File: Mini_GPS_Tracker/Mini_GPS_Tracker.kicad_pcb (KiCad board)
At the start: 2 copper layers, 34 parts, among them J1 USB_C_Receptacle, J2 5-1814400-1, J3 XT60-M, SW1 SW_Push, U1 CH340E, U2 XBee_SMT, U3 MAX-8Q, U4 LD1117S33TR_SOT223, U5 MS5611-01BA, Y1 Crystal

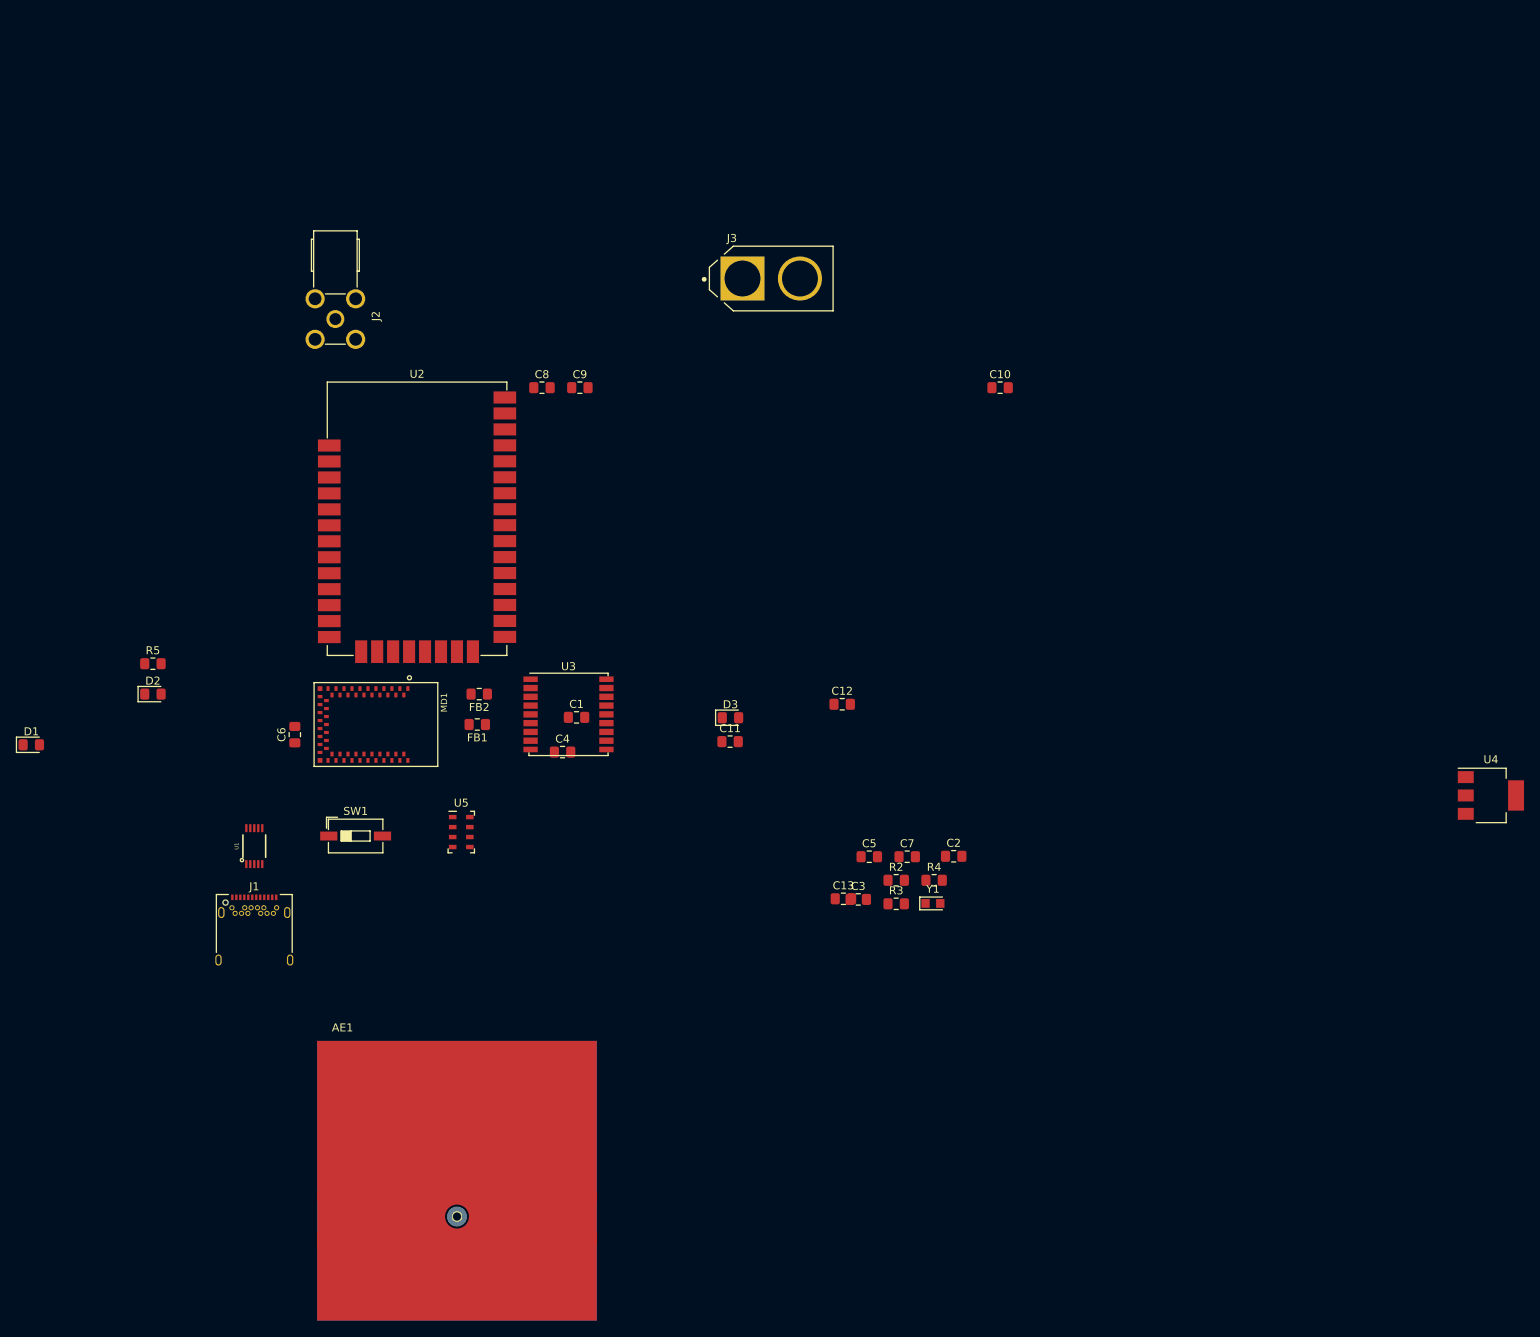
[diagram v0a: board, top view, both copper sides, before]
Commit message: worked on routing
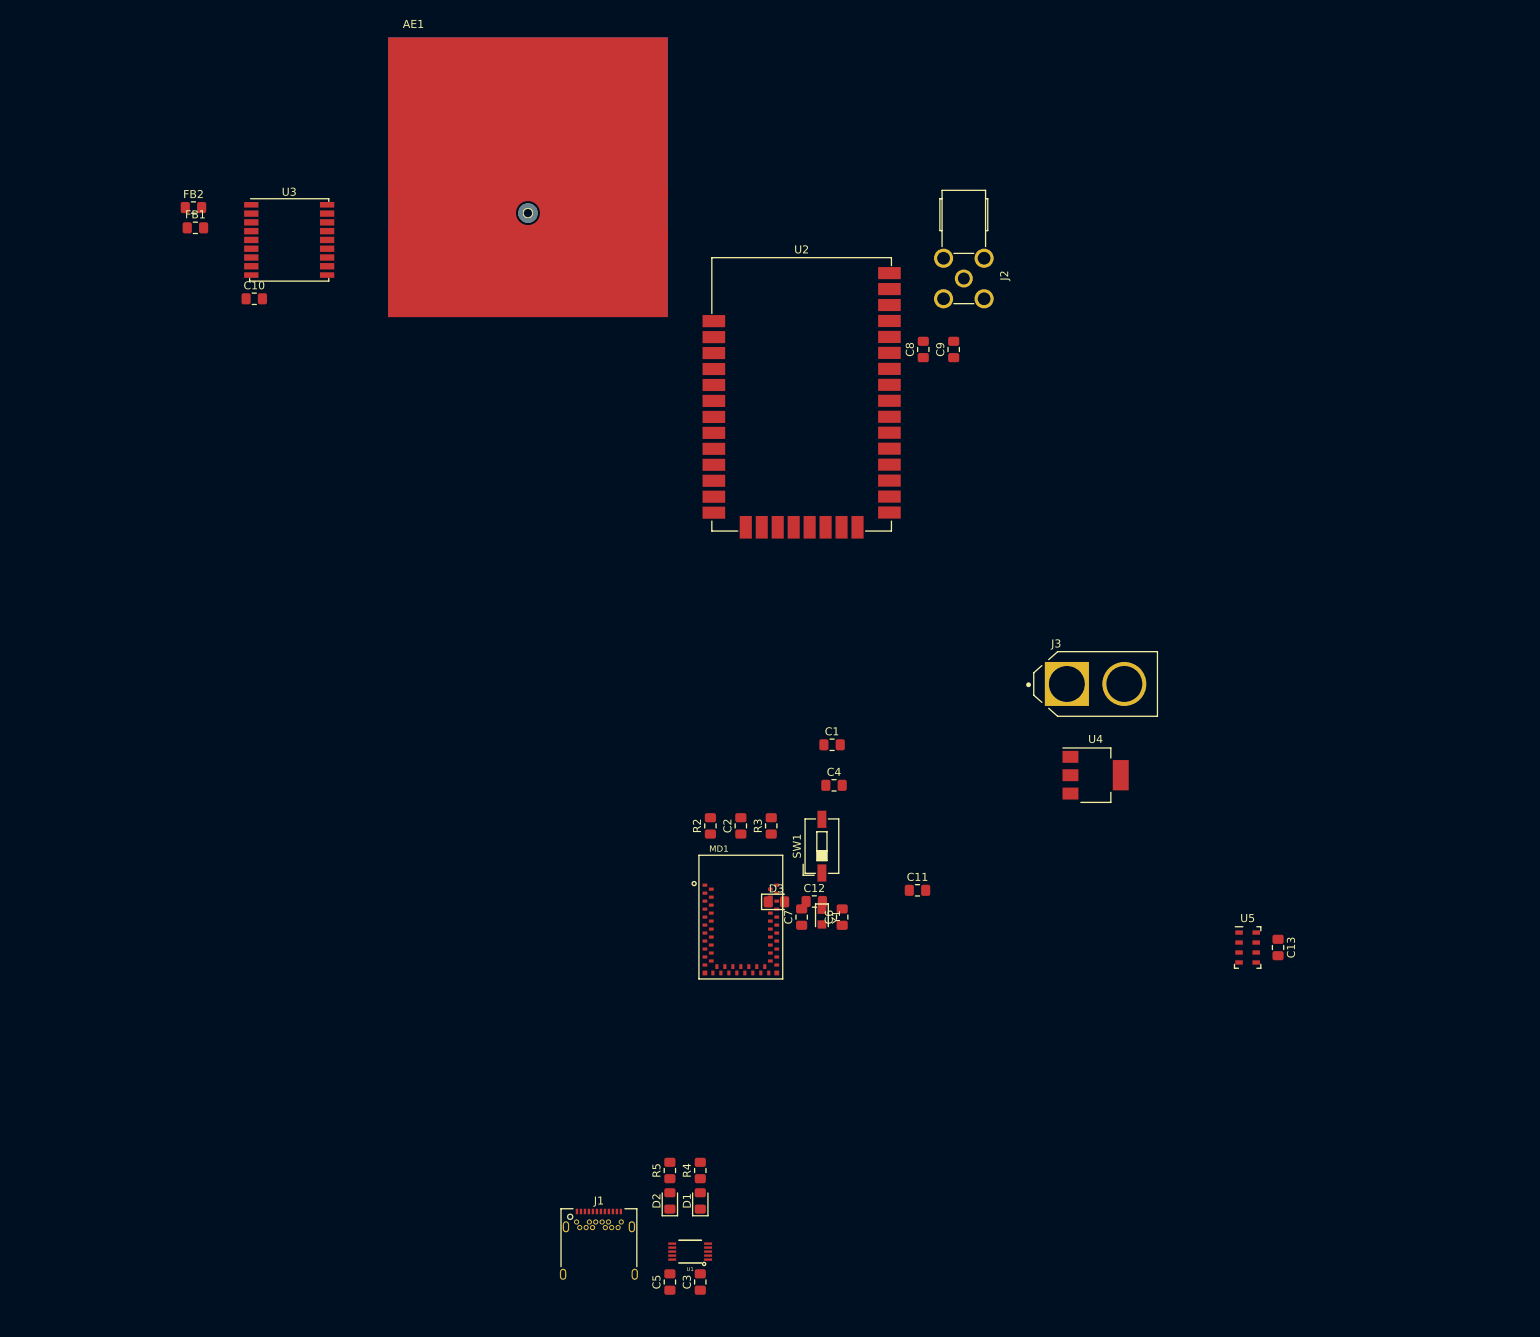
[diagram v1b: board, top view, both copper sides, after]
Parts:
- moved AE1 126.0 mm to (132.1, 20.3)
- moved D1 101.4 mm to (153.7, 148.6), turned to 90 degrees
- moved U5 99.6 mm to (222.2, 116.8)
- moved C10 94.1 mm to (97.8, 35.6)
- moved D2 90.7 mm to (149.9, 148.6), turned to 90 degrees
- moved R5 90.7 mm to (149.9, 144.8), turned to 90 degrees
- moved J2 78.9 mm to (186.7, 33.0)
- moved U1 74.6 mm to (152.4, 154.9), turned to 180 degrees
- moved C6 72.3 mm to (171.4, 113.0)
- moved FB1 71.6 mm to (90.4, 26.7), turned to 0 degrees
- moved FB2 70.7 mm to (90.2, 24.1), turned to 0 degrees
- moved U3 69.0 mm to (102.2, 28.2)
- moved J3 65.1 mm to (203.2, 83.8)
- moved C5 58.9 mm to (149.9, 158.8), turned to 90 degrees
- moved SW1 58.4 mm to (168.9, 104.1), turned to 90 degrees
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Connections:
- MD1 pad 12: Net-(MD1-Pad12) -> Pressure_SCL
- MD1 pad 23: Net-(MD1-Pad23) -> Pressure_SDA
